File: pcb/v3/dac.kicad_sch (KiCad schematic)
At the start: 63 parts, among them U14 CS43198, U15 CS43198, U16 OPA1622

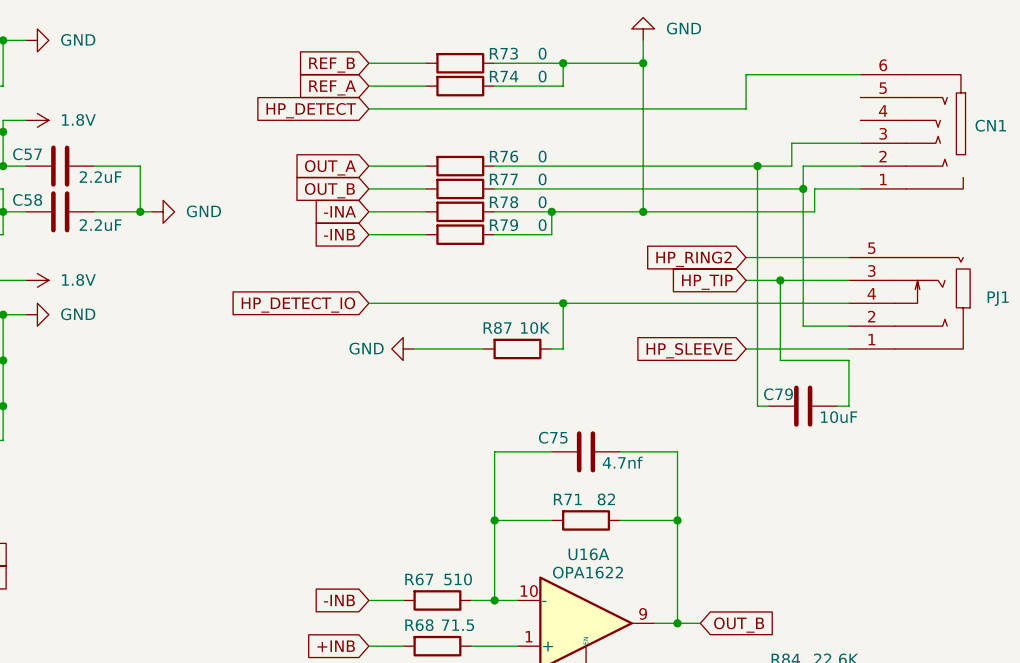
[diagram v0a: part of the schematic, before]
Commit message: up
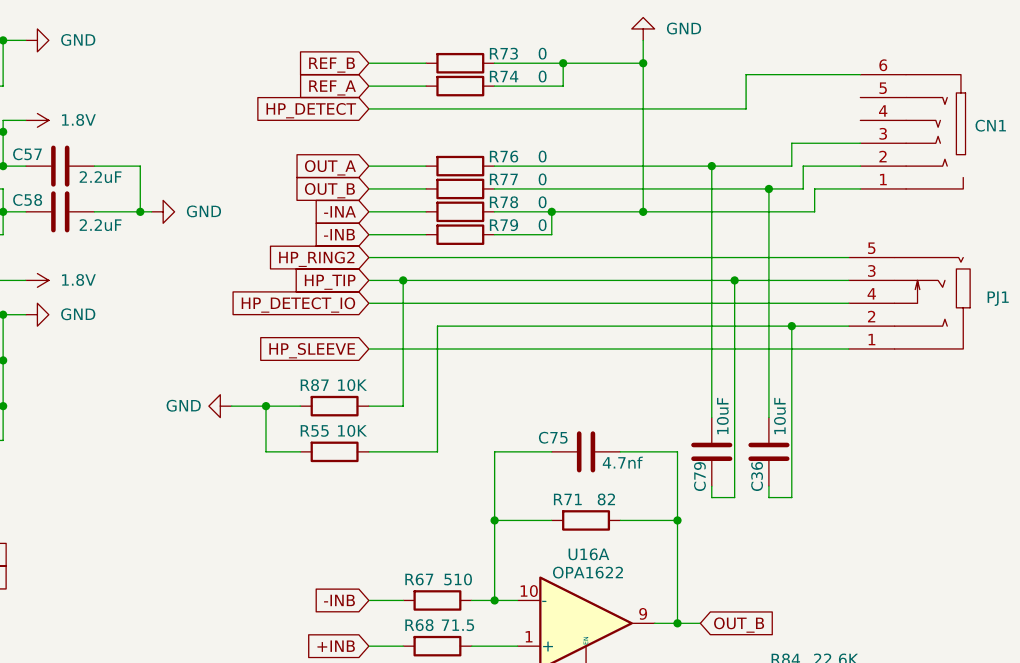
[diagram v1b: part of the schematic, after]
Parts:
- added C36: 10uF, Capacitor_SMD:C_0603_1608Metric_Pad1.08x0.95mm_HandSolder, symbol Device:C
- added R55: 10K, Capacitor_SMD:C_0402_1005Metric_Pad0.74x0.62mm_HandSolder, symbol Device:R
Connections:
- net GND: now also R55.2
- net HP_DETECT_IO: no longer R87.1
- net HP_TIP: now also C79.1, R87.1; no longer C79.2
- net at CN1.3, R76.1: now also C79.2; no longer C79.1
- net at CN1.2, R77.1: now also C36.2; no longer PJ1.2
- new net: C36.1, PJ1.2, R55.1
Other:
- moved on the sheet: C79, R87
